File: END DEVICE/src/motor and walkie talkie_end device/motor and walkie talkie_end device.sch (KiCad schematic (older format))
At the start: 14 parts, among them J1 ICSP, J2 FTDI_CONN, SW3 SW_Push, U1 ATmega328P-MU, Y1 16MHz

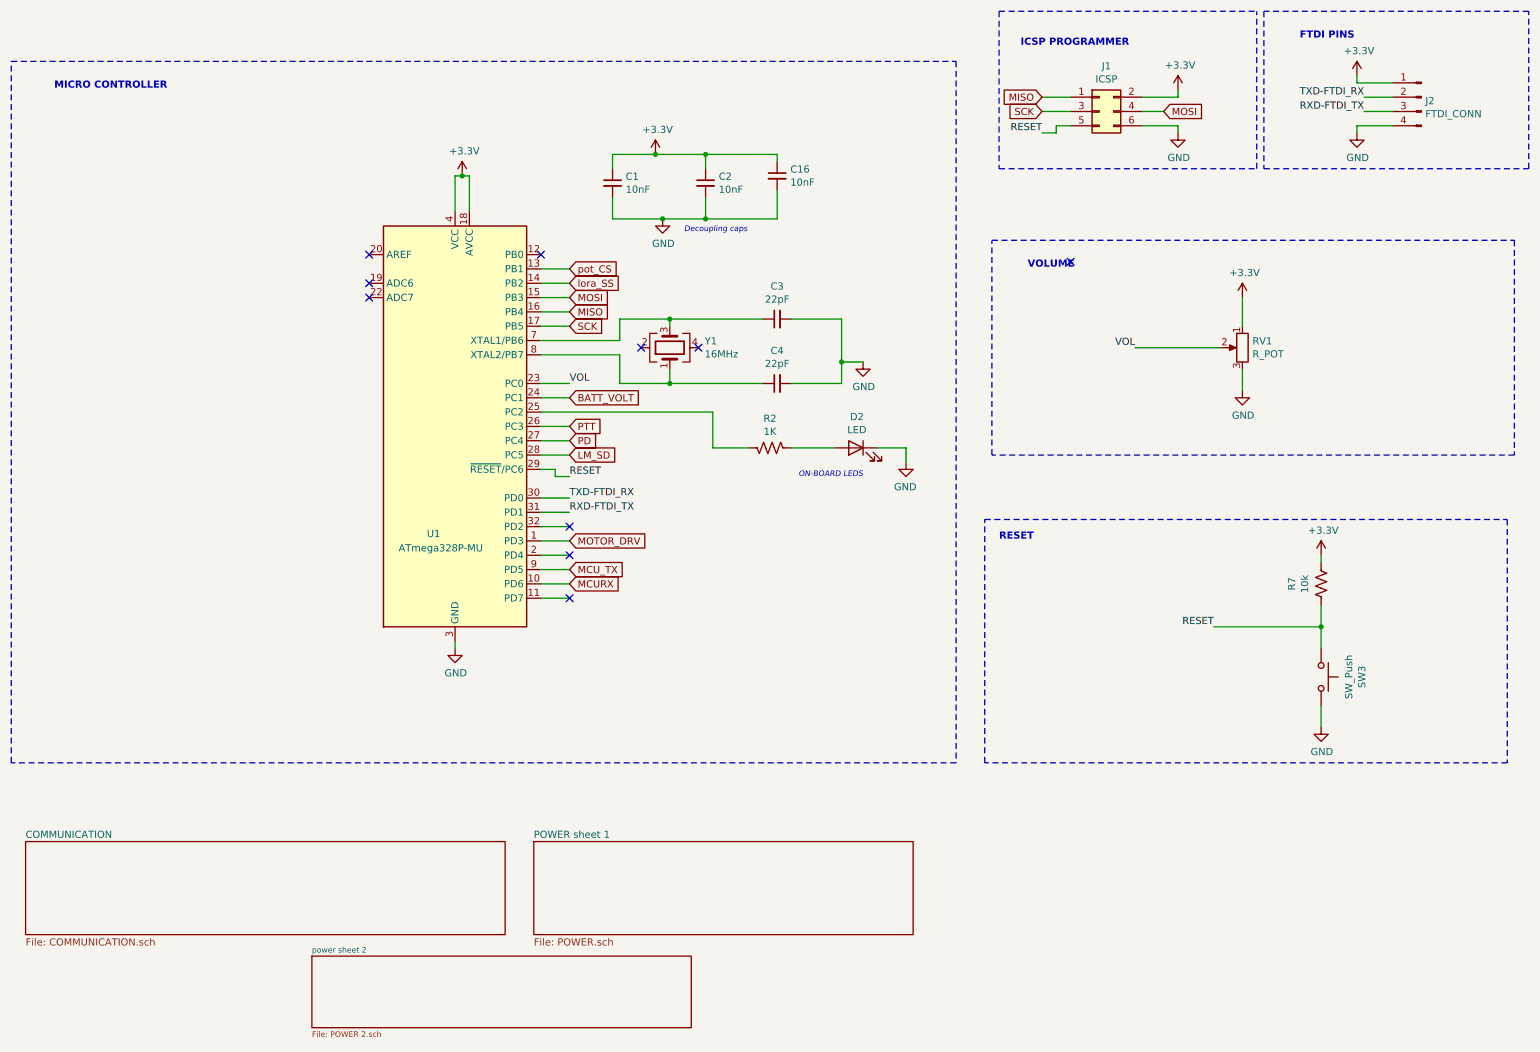
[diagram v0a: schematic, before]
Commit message: 90% complete and. PCB done with tracks and design rules verified as well as dimensions
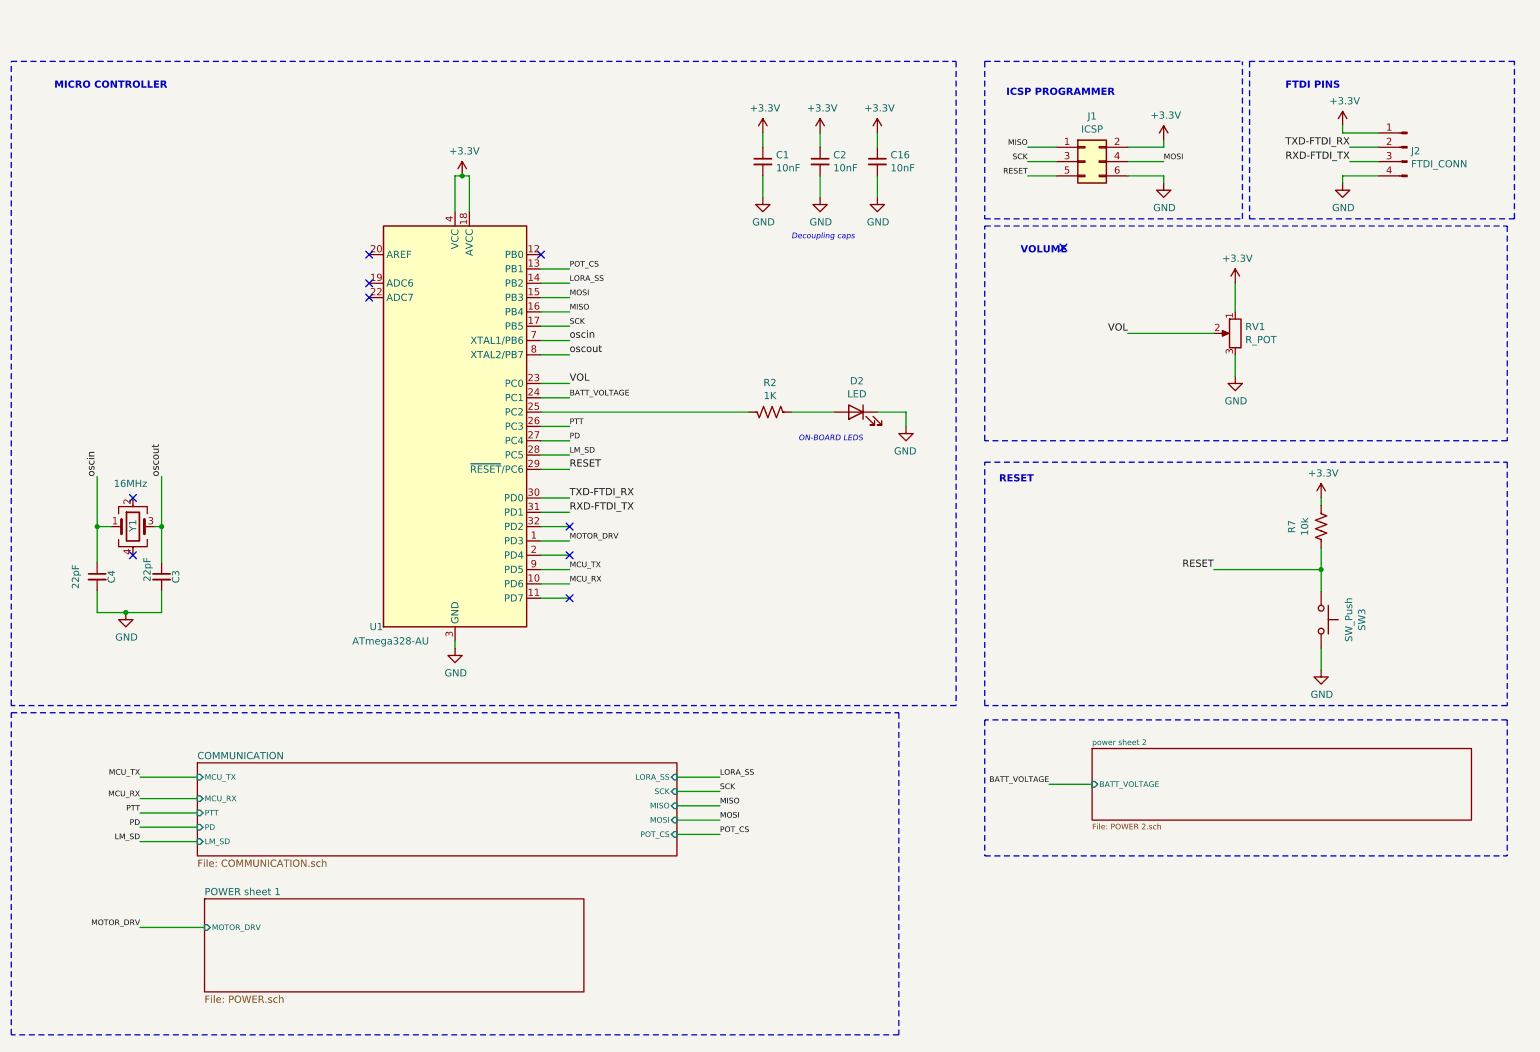
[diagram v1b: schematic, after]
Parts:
- removed U1: ATmega328P-MU, Package_DFN_QFN:QFN-32-1EP_5x5mm_P0.5mm_EP3.1x3.1mm, symbol MCU_Microchip_ATmega:ATmega328P-MU
- added U1: ATmega328-AU, Package_QFP:TQFP-32_7x7mm_P0.8mm, symbol MCU_Microchip_ATmega:ATmega328-AU
- RV1: footprint Potentiometer_THT:Potentiometer_Piher_PC-16_Single_Horizontal -> Potentiometer_THT:Potentiometer_Vishay_148-149_Single_Horizontal
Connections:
- net +3V3: now also U1.18 (AVCC), U1.4 (VCC), U1.6 (VCC)
- net GND: now also U1.21 (GND), U1.3 (GND), U1.5 (GND)
- net LM_SD: now also U1.28 (PC5)
- net MCU_TX: now also U1.9 (PD5)
- net MISO: now also U1.16 (PB4)
- net MOSI: now also U1.15 (PB3)
- net MOTOR_DRV: now also U1.1 (PD3)
- net PD: now also U1.27 (PC4)
- net PTT: now also U1.26 (PC3)
- net RESET: now also U1.29 (~RESET~/PC6)
- net RXD-FTDI_TX: now also U1.31 (PD1)
- net SCK: now also U1.17 (PB5)
- net TXD-FTDI_RX: now also U1.30 (PD0)
- net VOL: now also U1.23 (PC0)
- net at R2.1: now also U1.25 (PC2)
- net oscout: now reaches C3.1, Y1.3
- net oscout: now also U1.8 (XTAL2/PB7)
- net oscin: now reaches C4.1, Y1.1
- net oscin: now also U1.7 (XTAL1/PB6)
- new net BATT_VOLTAGE: U1.24 (PC1)
- new net LORA_SS: U1.14 (PB2)
- new net MCU_RX: U1.10 (PD6)
- new net POT_CS: U1.13 (PB1)
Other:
- moved on the sheet: C1, C2, C3, C4, D2, J1, J2, R2, R7, RV1, SW3, Y1
